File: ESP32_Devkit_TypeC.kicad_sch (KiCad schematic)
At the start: 57 parts, among them J1 USB_C_Receptacle_USB2.0, J2 Conn_01x19, J3 Conn_01x19, Q1 SS8050, Q2 SS8050, SW1 EN, SW2 BOOT, U1 MP2259, U2 CH340C, U3 ESP32-PICO-D4, Y1 12MHz

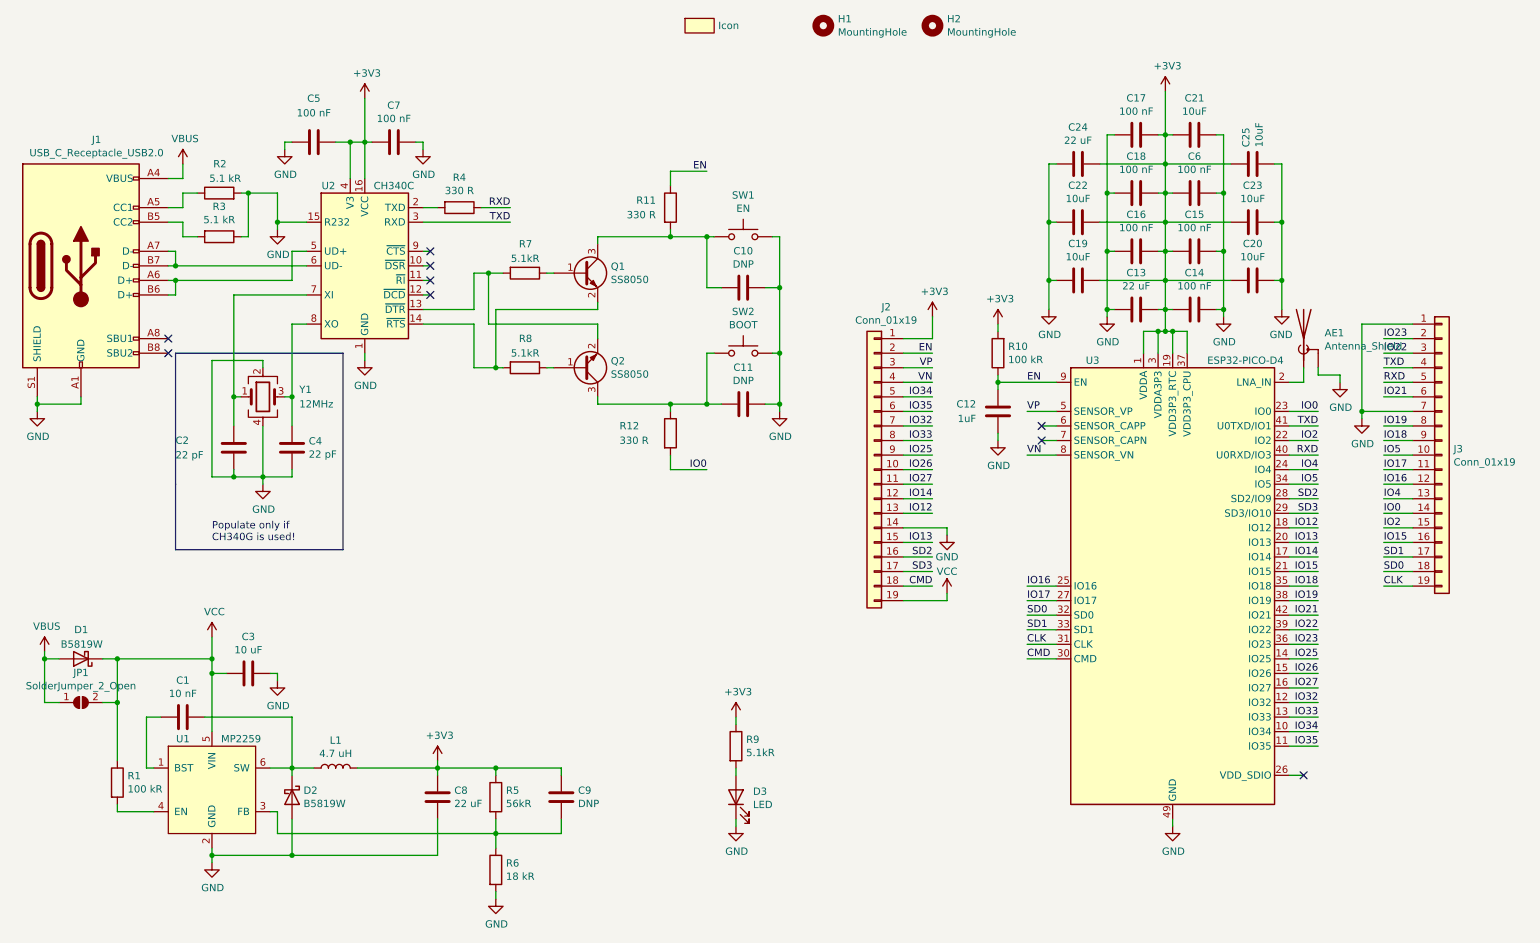
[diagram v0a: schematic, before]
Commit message: updated documentation
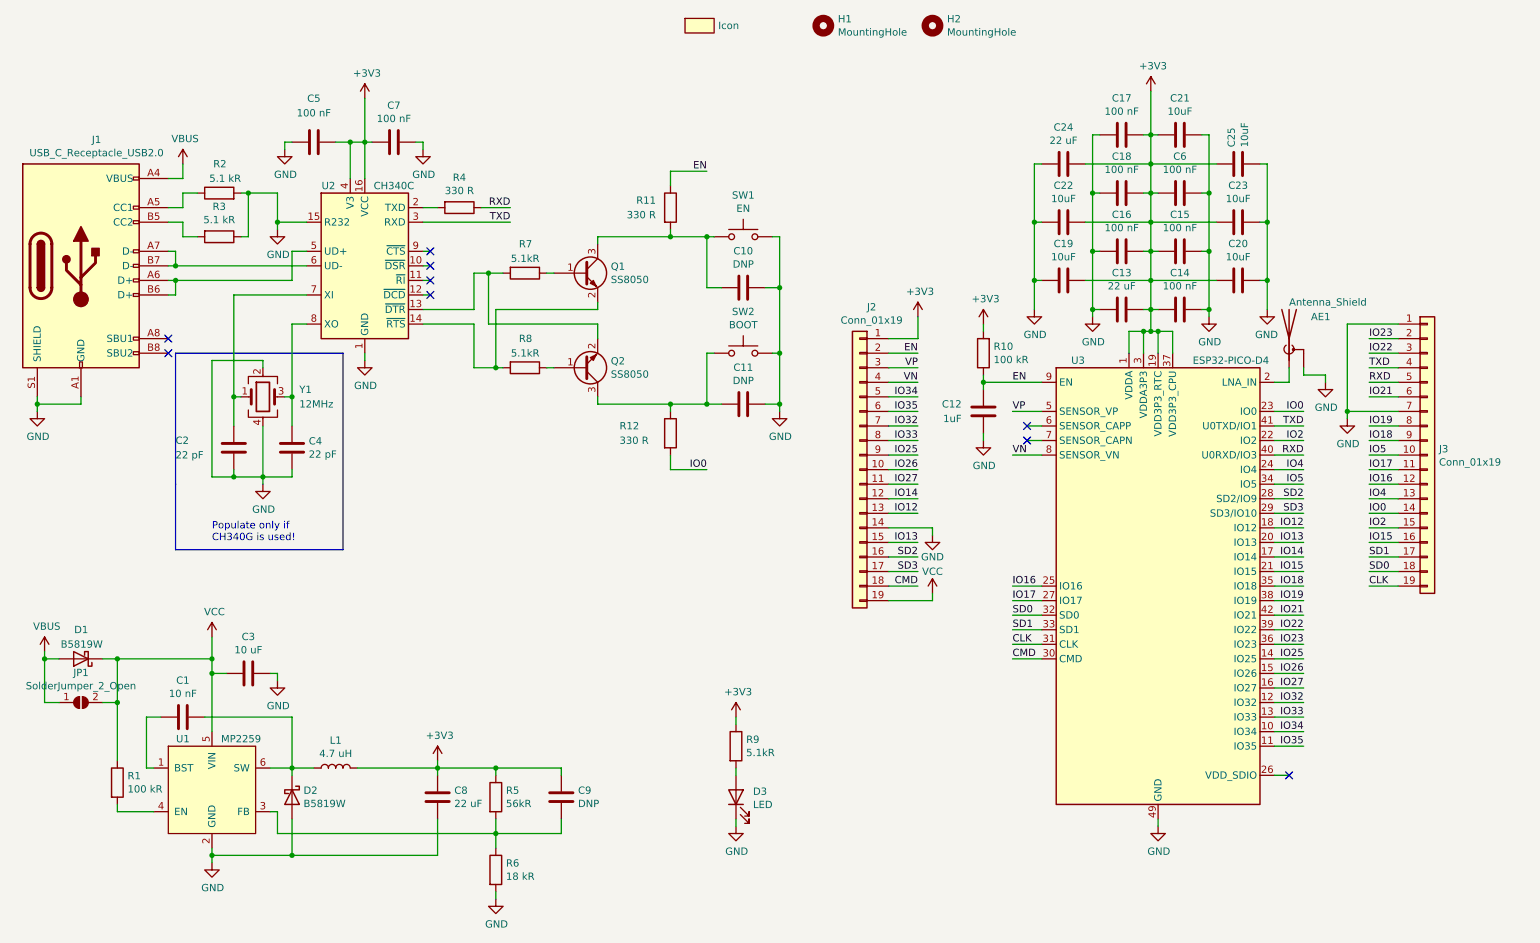
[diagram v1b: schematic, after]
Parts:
- AE1, C10, C11, C9, H1, H2, I2, JP1: now left out of the parts list
- J1: footprint Moucha_Connectors:USBC_Receptacle_TYPE-C-31-M-12 -> Connector_USB:USB_C_Receptacle_HRO_TYPE-C-31-M-12
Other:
- moved on the sheet: AE1, C12, C13, C14, C15, C16, C17, C18, C19, C20, C21, C22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
